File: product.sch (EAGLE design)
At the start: 0 parts

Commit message: work in progress
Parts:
- added C1, C2, C4, C5: 1uF, SparkFun-Capacitors:CAP0805
- added C3: 104, SparkFun-Capacitors:CAP0805
- added C6: 0.1uF, SparkFun-Passives:CAP0402-CAP
- added C7, C8: 16pF, SparkFun:CAP0805
- added Q2: 16MHz, crystal:CRYSTALCTS406
- added R1: 390k/560k, SparkFun-Resistors:RESISTOR0805-RES
- added R2: 100k, SparkFun-Passives:RESISTOR0402-RES
- added S1, S2: SWITCH-MOMENTARY-2SMD, SparkFun-Electromechanical:SWITCH-MOMENTARY-2SMD
- added U$1: LM4F120H5QR, stellaris:LM4F120H5QR
- added U1: ATSHA204-TSU, SparkFun-DigitalIC:ATSHA204-TSU
- added U2: (no value), SparkFun-Connectors:USB-AB
- added U3: (no value), microbuilder:DISP_OLED_UG-2864HSWEG010.96"
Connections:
- new net +3V3: C3.1, C4.1, C6.1, R2.2, S1.2, S2.2, U$1.VDD, U1.VCC, U3.VDD
- new net +5V: U2.VBUS
- new net GND: C3.2, C4.2, C5.2, C6.2, C7.2, C8.2, R1.2, U$1.GND, U1.GND, U2.GND, U3.BS0, U3.BS1, U3.BS2, U3.NC(GND)@1, U3.NC(GND)@2, U3.VLSS
- new net N$1: U$1.PA5/SSI0TX, U3.D1/SPI_SDIN/I2C_SDA
- new net N$10: C1.1, U3.C2P
- new net N$11: C2.1, U3.C1P
- new net N$12: C1.2, U3.C2N
- new net N$13: C2.2, U3.C1N
- new net N$14: S2.1, U$1.PF1
- new net N$15: S1.1, U$1.PF0
- new net N$2: U$1.PE0, U3./CS
- new net N$3: U$1.PD4, U2.D-
- new net N$4: U$1.PE2, U3.DC/I2C_SA0
- new net N$5: U$1.PA2/SSI0CLK, U3.D0/SPI_SCLK/I2C_SCK
- new net N$6: C5.1, U3.VCOMH
- new net N$7: U$1.PD5, U2.D+
- new net N$8: U$1.PE1, U3./RES
- new net N$9: R1.1, U3.IREF
- new net SDA: R2.1, U$1.PB0, U1.SDA
- new net XTAL1: C7.1, Q2.1, U$1.OSC0
- new net XTAL2: C8.1, Q2.2, U$1.OSC1

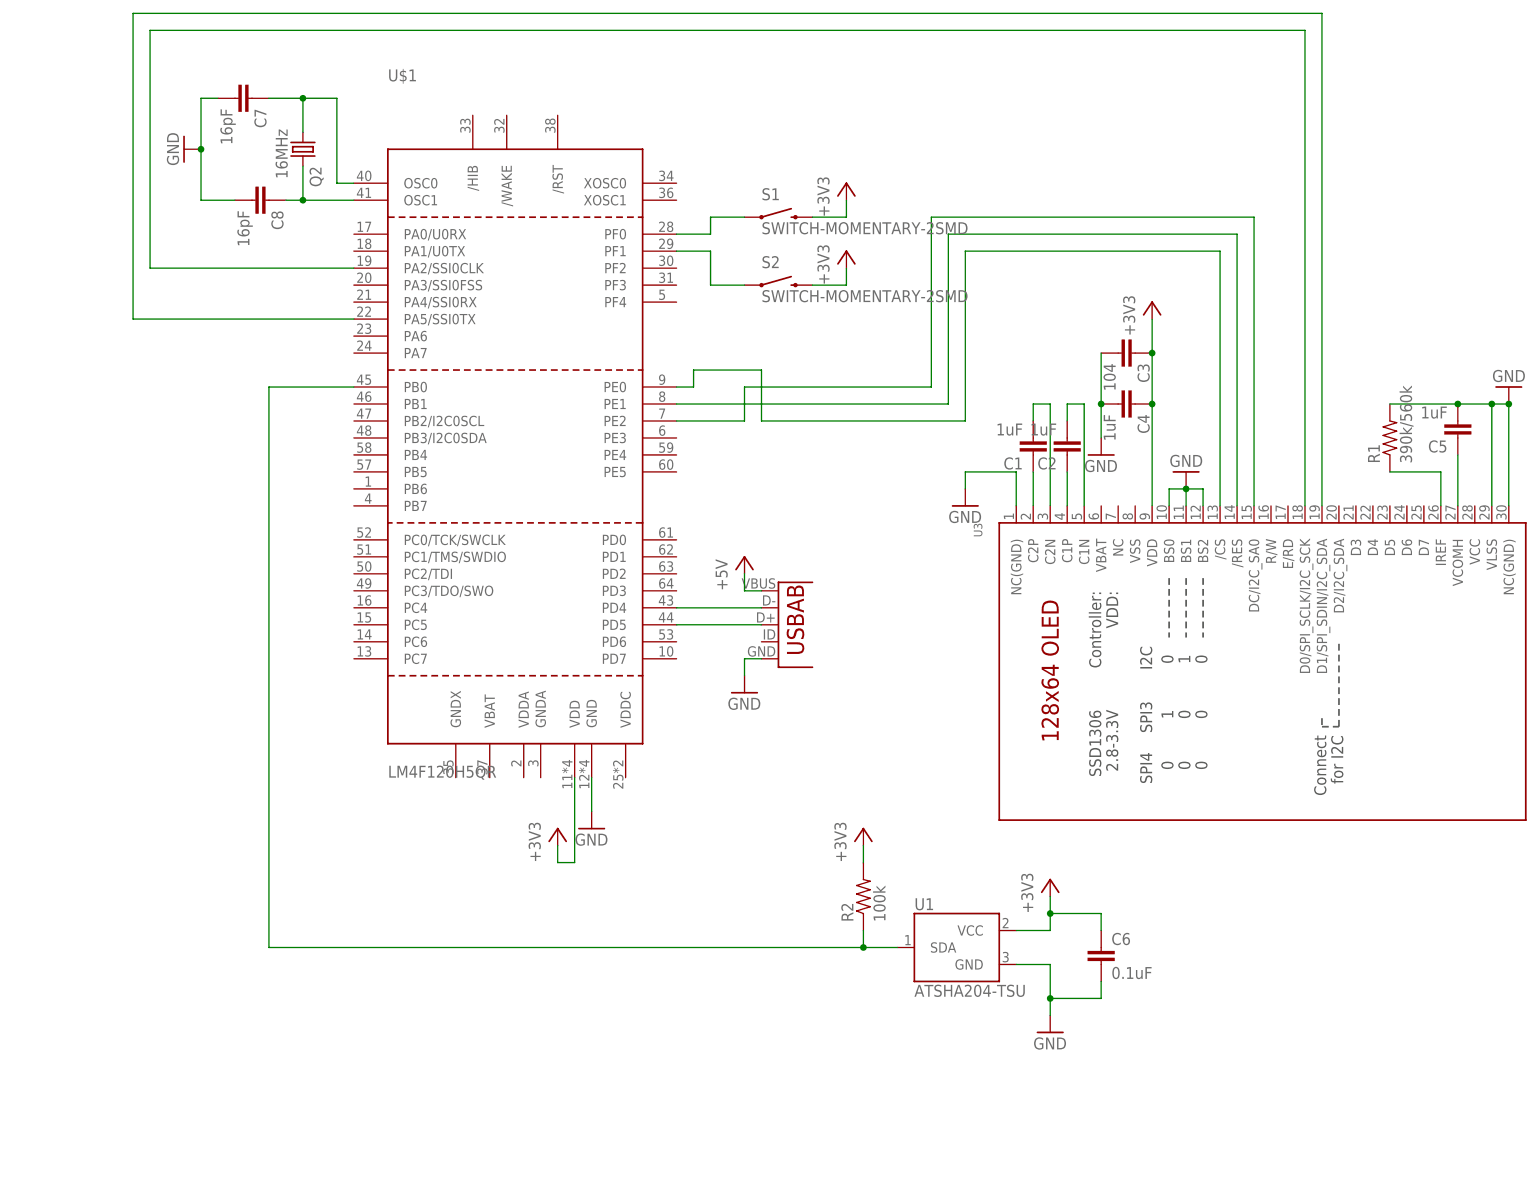
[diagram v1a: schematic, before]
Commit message: work on product scheme
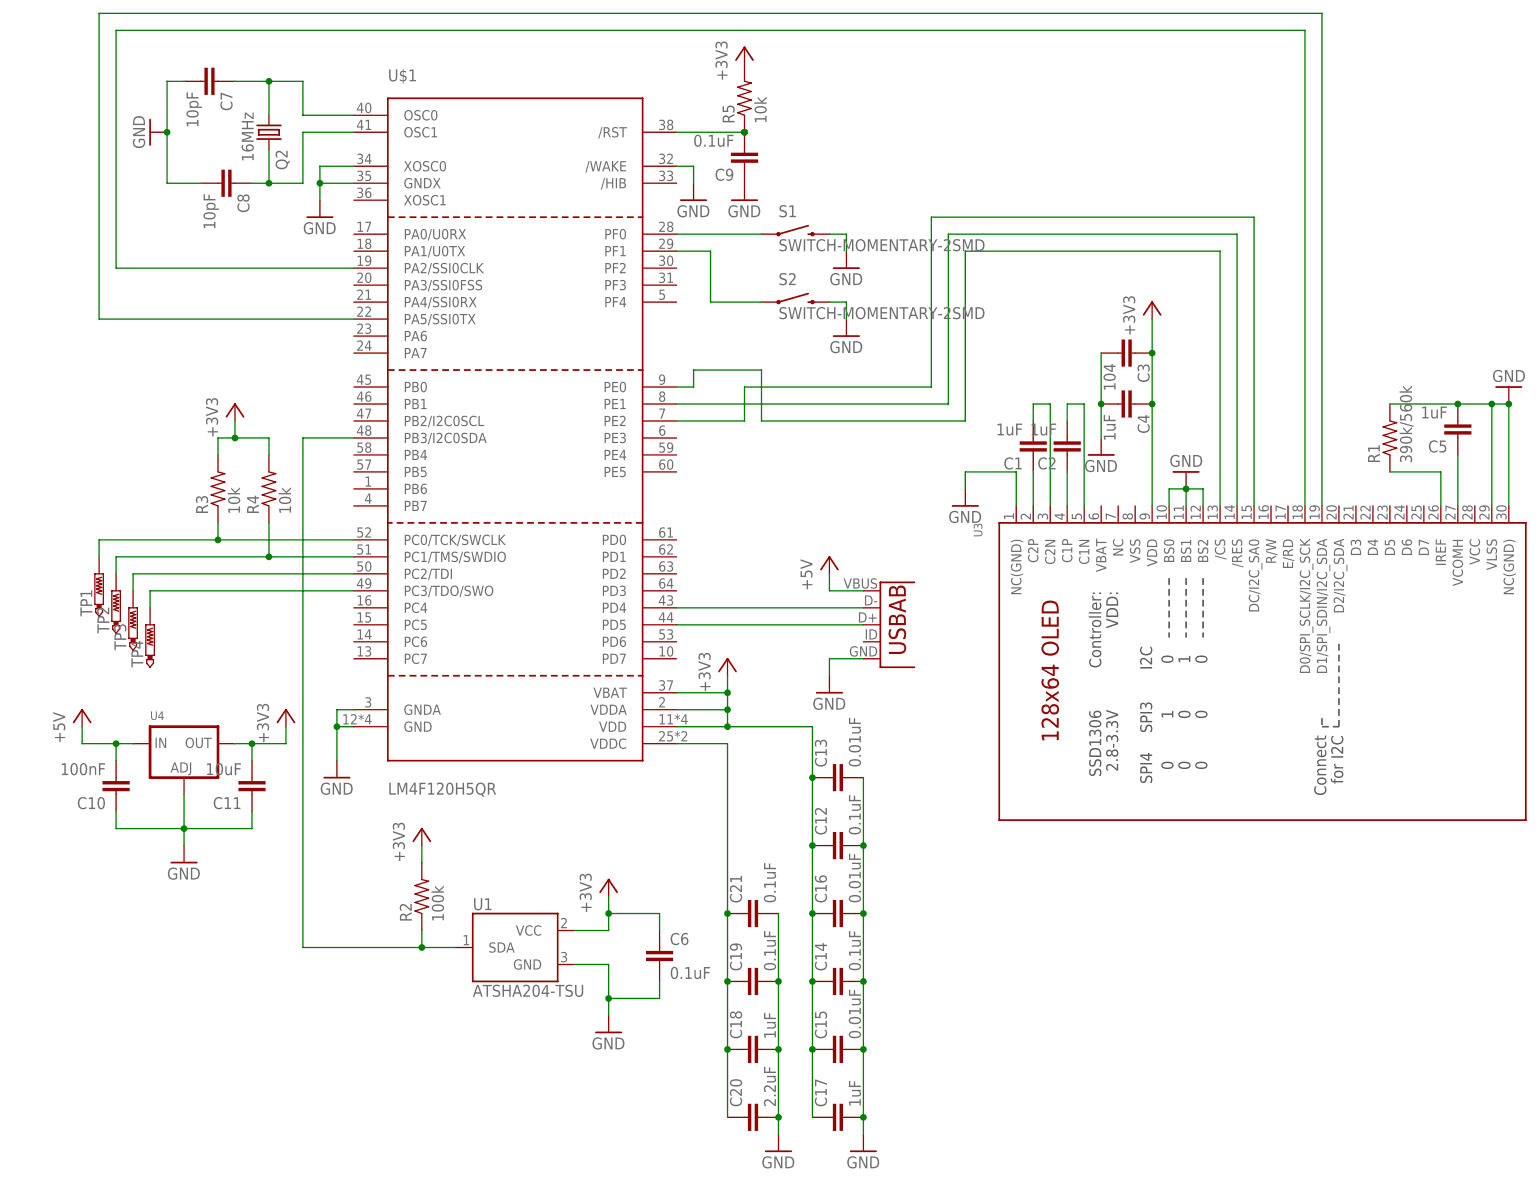
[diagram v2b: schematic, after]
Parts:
- added C10: 100nF, SparkFun-Capacitors:CAP0805
- added C11: 10uF, SparkFun-Capacitors:CAP0805
- added C12, C14, C19, C21: 0.1uF, SparkFun-Passives:CAP0402-CAP
- added C13, C15, C16: 0.01uF, SparkFun-Passives:CAP0402-CAP
- added C17, C18: 1uF, SparkFun-Passives:CAP0402-CAP
- added C20: 2.2uF, SparkFun-Passives:CAP0402-CAP
- added C9: 0.1uF, SparkFun:CAP0805
- added R3, R4, R5: 10k, SparkFun-Passives:RESISTOR0402-RES
- added TP1, TP2, TP3, TP4: PTR1TP10R, testpad:PTR1TP10R
- added U4: (no value), microbuilder:LM1117SOT223-REFLOW
- C7, C8: value 16pF -> 10pF
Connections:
- new net N$16: R4.1, TP2.TP, U$1.PC1/TMS/SWDIO
- new net N$17: R3.1, TP1.TP, U$1.PC0/TCK/SWCLK
- new net N$19: TP3.TP, U$1.PC2/TDI
- new net N$20: TP4.TP, U$1.PC3/TDO/SWO
- new net N$21: C9.2, R5.1, U$1./RST
- new net N$23: C18.1, C19.1, C20.1, C21.1, U$1.VDDC
- net +3V3: now also C11.2, C12.1, C13.1, C14.1, C15.1, C16.1, C17.1, R3.2, R4.2, R5.2, U$1.VBAT, U$1.VDDA, U4.OUT; no longer S1.2, S2.2
- net +5V: now also C10.2, U4.IN
- net GND: now also C10.1, C11.1, C12.2, C13.2, C14.2, C15.2, C16.2, C17.2, C18.2, C19.2, C20.2, C21.2, C9.1, S1.2, S2.2, U$1./WAKE, U$1.GNDA, U$1.GNDX, U$1.XOSC0, U4.ADJ
- net SDA: now also U$1.PB3/I2C0SDA; no longer U$1.PB0
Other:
- moved on the sheet: C6, C7, C8, Q2, R2, S1, S2, U$1, U1

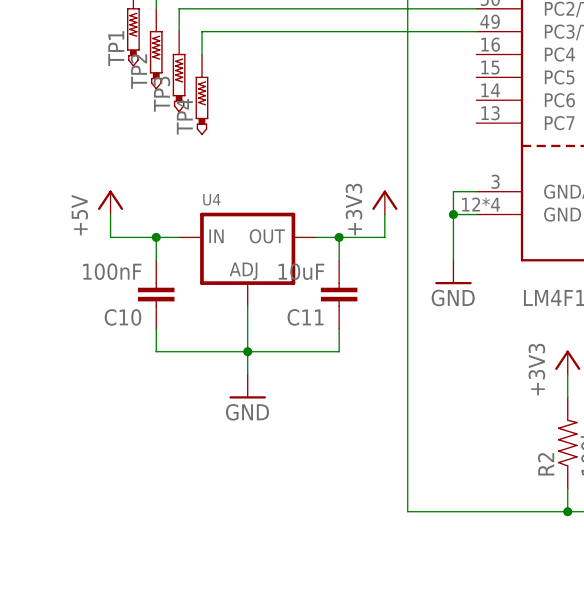
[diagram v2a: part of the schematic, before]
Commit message: wip
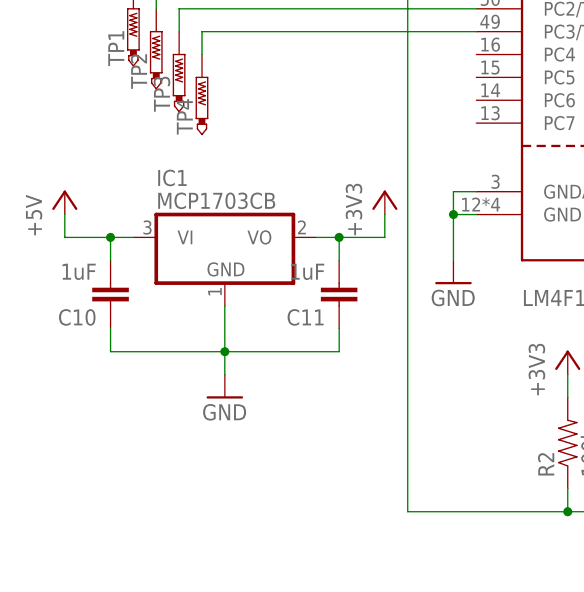
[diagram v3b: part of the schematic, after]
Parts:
- removed U4: (no value), microbuilder:LM1117SOT223-REFLOW
- added IC1: MCP1703CB, linear:MCP1703CB
- C1, C2, C3, C4, C5: device SparkFun-Capacitors:CAP0805 -> SparkFun-Passives:CAP0402-CAP
- C10: value 100nF -> 1uF; device SparkFun-Capacitors:CAP0805 -> SparkFun-Passives:CAP0402-CAP
- C11: value 10uF -> 1uF; device SparkFun-Capacitors:CAP0805 -> SparkFun-Passives:CAP0402-CAP
- C7, C8, C9: device SparkFun:CAP0805 -> SparkFun-Passives:CAP0402-CAP
- R1: device SparkFun-Resistors:RESISTOR0805-RES -> SparkFun-Passives:RESISTOR0402-RES
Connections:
- net +3V3: now also IC1.VO; no longer U4.OUT
- net +5V: now also IC1.VI; no longer U4.IN
- net GND: now also IC1.GND; no longer U4.ADJ
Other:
- moved on the sheet: C10
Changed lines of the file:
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@@
 <part name="GND3" library="supply1" deviceset="GND" device=""/>
 <part name="GND5" library="supply1" deviceset="GND" device=""/>
-<part name="C1" library="SparkFun-Capacitors" deviceset="CAP" device="0805" value="1uF"/>
-<part name="C2" library="SparkFun-Capacitors" deviceset="CAP" device="0805" value="1uF"/>
-<part name="C3" library="SparkFun-Capacitors" deviceset="CAP" device="0805" value="104"/>
-<part name="C4" library="SparkFun-Capacitors" deviceset="CAP" device="0805" value="1uF"/>
+<part name="C1" library="SparkFun-Passives" deviceset="CAP" device="0402-CAP" value="1uF"/>
+<part name="C2" library="SparkFun-Passives" deviceset="CAP" device="0402-CAP" value="1uF"/>
+<part name="C3" library="SparkFun-Passives" deviceset="CAP" device="0402-CAP" value="104"/>
+<part name="C4" library="SparkFun-Passives" deviceset="CAP" device="0402-CAP" value="1uF"/>
 <part name="GND6" library="supply1" deviceset="GND" device=""/>
-<part name="C5" library="SparkFun-Capacitors" deviceset="CAP" device="0805" value="1uF"/>
-<part name="R1" library="SparkFun-Resistors" deviceset="RESISTOR" device="0805-RES" value="390k/560k"/>
+<part name="C5" library="SparkFun-Passives" deviceset="CAP" device="0402-CAP" value="1uF"/>
+<part name="R1" library="SparkFun-Passives" deviceset="RESISTOR" device="0402-RES" value="390k/560k"/>
 <part name="P+1" library="supply1" deviceset="+5V" device=""/>
 <part name="GND1" library="supply1" deviceset="GND" device=""/>
@@
 <part name="+3V7" library="supply1" deviceset="+3V3" device=""/>
 <part name="Q2" library="crystal" deviceset="CRYSTAL" device="CTS406" value="16MHz"/>
-<part name="C7" library="SparkFun" deviceset="CAP" device="0805" value="10pF"/>
-<part name="C8" library="SparkFun" deviceset="CAP" device="0805" value="10pF"/>
+<part name="C7" library="SparkFun-Passives" deviceset="CAP" device="0402-CAP" value="10pF"/>
+<part name="C8" library="SparkFun-Passives" deviceset="CAP" device="0402-CAP" value="10pF"/>
 <part name="GND7" library="SparkFun" deviceset="GND" device=""/>
 <part name="GND9" library="supply1" deviceset="GND" device=""/>
 <part name="GND10" library="supply1" deviceset="GND" device=""/>
-<part name="C9" library="SparkFun" deviceset="CAP" device="0805" value="0.1uF"/>
-<part name="U4" library="microbuilder" deviceset="LM1117" device="SOT223-REFLOW"/>
+<part name="C9" library="SparkFun-Passives" deviceset="CAP" device="0402-CAP" value="0.1uF"/>
 <part name="P+2" library="supply1" deviceset="+5V" device=""/>
 <part name="GND11" library="supply1" deviceset="GND" device=""/>
 <part name="+3V1" library="supply1" deviceset="+3V3" device=""/>
-<part name="C10" library="SparkFun-Capacitors" deviceset="CAP" device="0805" value="100nF"/>
-<part name="C11" library="SparkFun-Capacitors" deviceset="CAP" device="0805" value="10uF"/>
+<part name="C10" library="SparkFun-Passives" deviceset="CAP" device="0402-CAP" value="1uF"/>
+<part name="C11" library="SparkFun-Passives" deviceset="CAP" device="0402-CAP" value="1uF"/>
 <part name="GND12" library="supply1" deviceset="GND" device=""/>
 <part name="GND13" library="supply1" deviceset="GND" device=""/>
@@
 <attribute name="TP_SIGNAL_NAME" value=""/>
 </part>
+<part name="IC1" library="linear" deviceset="MCP1703" device="CB"/>
 </parts>
 <sheets>
@@
 <instance part="GND10" gate="1" x="48.26" y="91.44"/>
 <instance part="C9" gate="G$1" x="55.88" y="99.06" rot="R180"/>
-<instance part="U4" gate="G$1" x="-27.94" y="10.16"/>
-<instance part="P+2" gate="1" x="-43.18" y="15.24"/>
-<instance part="GND11" gate="1" x="-27.94" y="-7.62"/>
+<instance part="P+2" gate="1" x="-48.26" y="15.24"/>
+<instance part="GND11" gate="1" x="-30.48" y="-7.62"/>
 <instance part="+3V1" gate="G$1" x="-12.7" y="15.24"/>
-<instance part="C10" gate="G$1" x="-38.1" y="5.08" rot="R180"/>
+<instance part="C10" gate="G$1" x="-43.18" y="5.08" rot="R180"/>
 <instance part="C11" gate="G$1" x="-17.78" y="5.08" rot="R180"/>
 <instance part="GND12" gate="1" x="71.12" y="81.28"/>
@@
 <instance part="TP3" gate="G$1" x="-35.56" y="30.48"/>
 <instance part="TP4" gate="G$1" x="-33.02" y="27.94"/>
+<instance part="IC1" gate="G$1" x="-30.48" y="10.16"/>
 </instances>
 <busses>
@@
 <wire x1="-17.78" y1="10.16" x2="-12.7" y2="10.16" width="0.1524" layer="91"/>
 <wire x1="-12.7" y1="10.16" x2="-12.7" y2="12.7" width="0.1524" layer="91"/>
-<pinref part="U4" gate="G$1" pin="OUT"/>
 <pinref part="C11" gate="G$1" pin="2"/>
 <wire x1="-17.78" y1="7.62" x2="-17.78" y2="10.16" width="0.1524" layer="91"/>
 <junction x="-17.78" y="10.16"/>
+<pinref part="IC1" gate="G$1" pin="VO"/>
 </segment>
 <segment>
@@
 </segment>
 <segment>
-<pinref part="U4" gate="G$1" pin="ADJ"/>
 <pinref part="GND11" gate="1" pin="GND"/>
-<wire x1="-27.94" y1="2.54" x2="-27.94" y2="-2.54" width="0.1524" layer="91"/>
-<wire x1="-27.94" y1="-2.54" x2="-27.94" y2="-5.08" width="0.1524" layer="91"/>
+<wire x1="-30.48" y1="2.54" x2="-30.48" y2="-2.54" width="0.1524" layer="91"/>
+<wire x1="-30.48" y1="-2.54" x2="-30.48" y2="-5.08" width="0.1524" layer="91"/>
 <pinref part="C11" gate="G$1" pin="1"/>
 <wire x1="-17.78" y1="0" x2="-17.78" y2="-2.54" width="0.1524" layer="91"/>
-<wire x1="-17.78" y1="-2.54" x2="-27.94" y2="-2.54" width="0.1524" layer="91"/>
-<junction x="-27.94" y="-2.54"/>
-<wire x1="-27.94" y1="-2.54" x2="-38.1" y2="-2.54" width="0.1524" layer="91"/>
+<wire x1="-17.78" y1="-2.54" x2="-30.48" y2="-2.54" width="0.1524" layer="91"/>
+<junction x="-30.48" y="-2.54"/>
+<wire x1="-30.48" y1="-2.54" x2="-43.18" y2="-2.54" width="0.1524" layer="91"/>
 <pinref part="C10" gate="G$1" pin="1"/>
-<wire x1="-38.1" y1="-2.54" x2="-38.1" y2="0" width="0.1524" layer="91"/>
+<wire x1="-43.18" y1="-2.54" x2="-43.18" y2="0" width="0.1524" layer="91"/>
+<pinref part="IC1" gate="G$1" pin="GND"/>
 </segment>
 <segment>
@@
 </segment>
 <segment>
-<pinref part="U4" gate="G$1" pin="IN"/>
 <pinref part="P+2" gate="1" pin="+5V"/>
-<wire x1="-35.56" y1="10.16" x2="-38.1" y2="10.16" width="0.1524" layer="91"/>
+<wire x1="-40.64" y1="10.16" x2="-43.18" y2="10.16" width="0.1524" layer="91"/>
 <pinref part="C10" gate="G$1" pin="2"/>
-<wire x1="-38.1" y1="10.16" x2="-43.18" y2="10.16" width="0.1524" layer="91"/>
-<wire x1="-43.18" y1="10.16" x2="-43.18" y2="12.7" width="0.1524" layer="91"/>
-<wire x1="-38.1" y1="10.16" x2="-38.1" y2="7.62" width="0.1524" layer="91"/>
-<junction x="-38.1" y="10.16"/>
-</segment>
-</net>
+<wire x1="-43.18" y1="10.16" x2="-48.26" y2="10.16" width="0.1524" layer="91"/>
+<wire x1="-48.26" y1="10.16" x2="-48.26" y2="12.7" width="0.1524" layer="91"/>
+<wire x1="-43.18" y1="10.16" x2="-43.18" y2="7.62" width="0.1524" layer="91"/>
+<junction x="-43.18" y="10.16"/>
+<pinref part="IC1" gate="G$1" pin="VI"/>
+</segment>
+</net>
